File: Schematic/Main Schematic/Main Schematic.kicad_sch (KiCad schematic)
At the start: 5 parts, among them J1 Conn_01x10_Pin, J2 Conn_01x24_Socket, J3 Conn_01x24_Socket, SW2 SW_Push

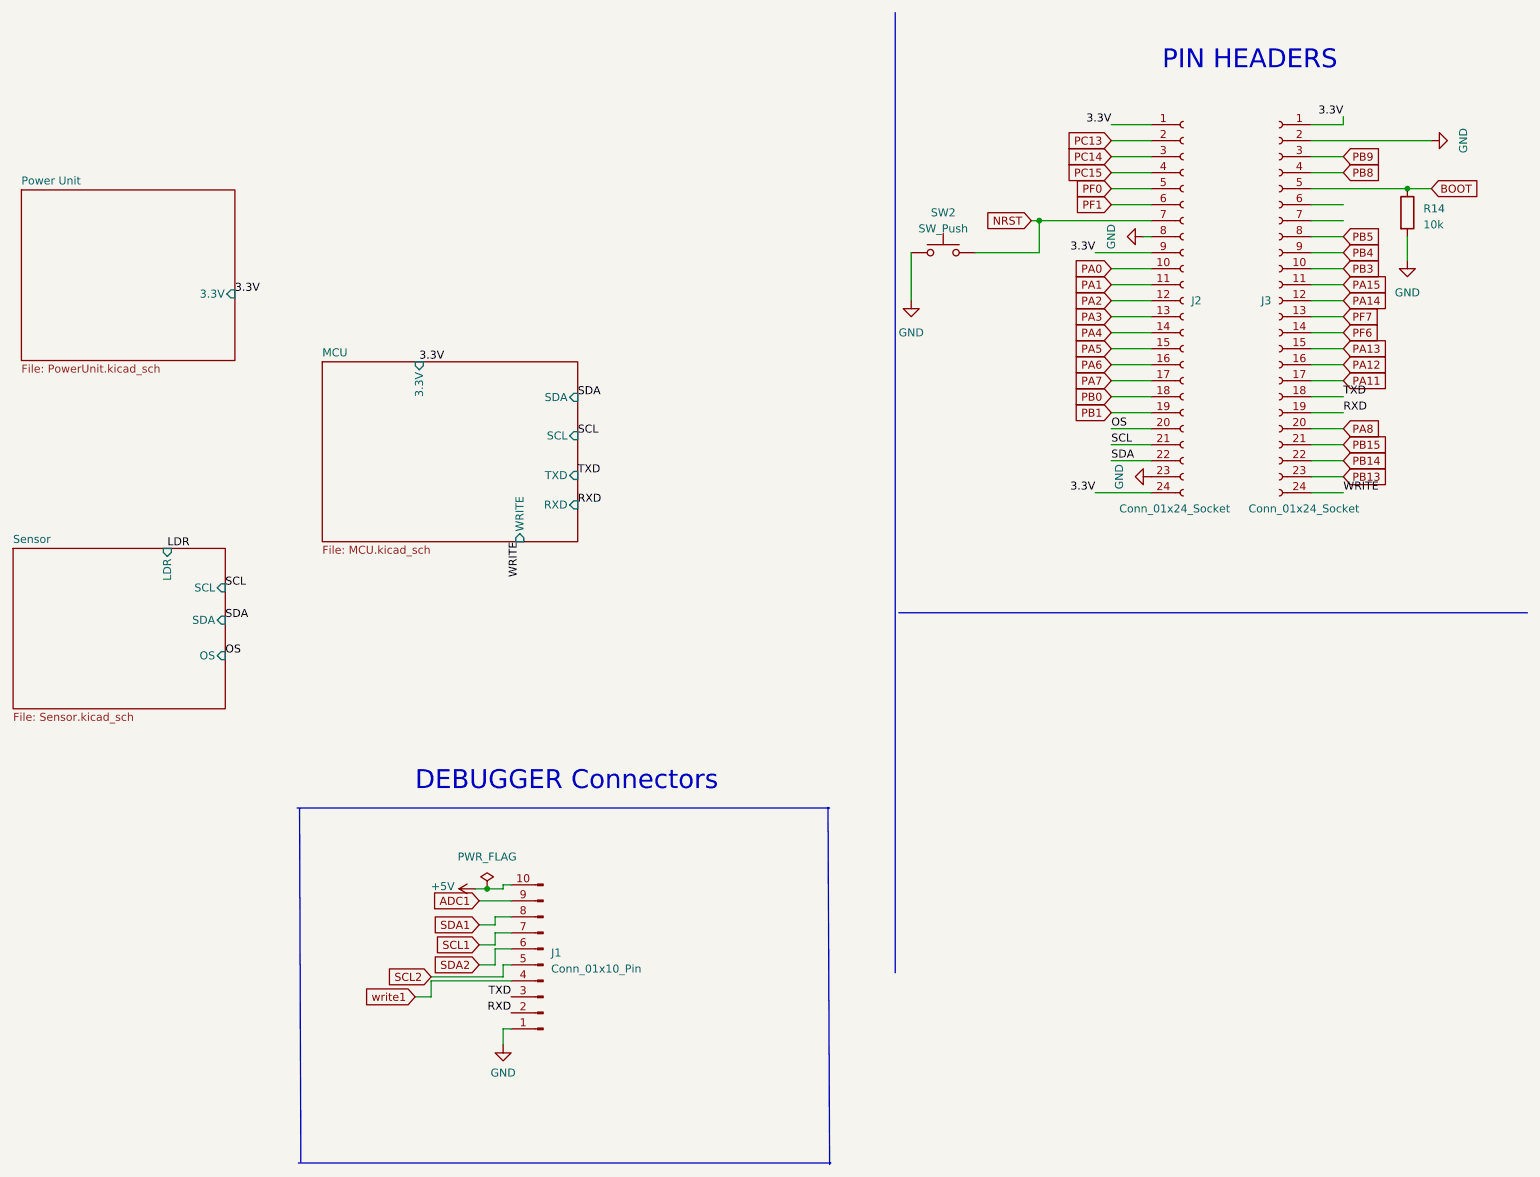
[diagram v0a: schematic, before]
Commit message: Update
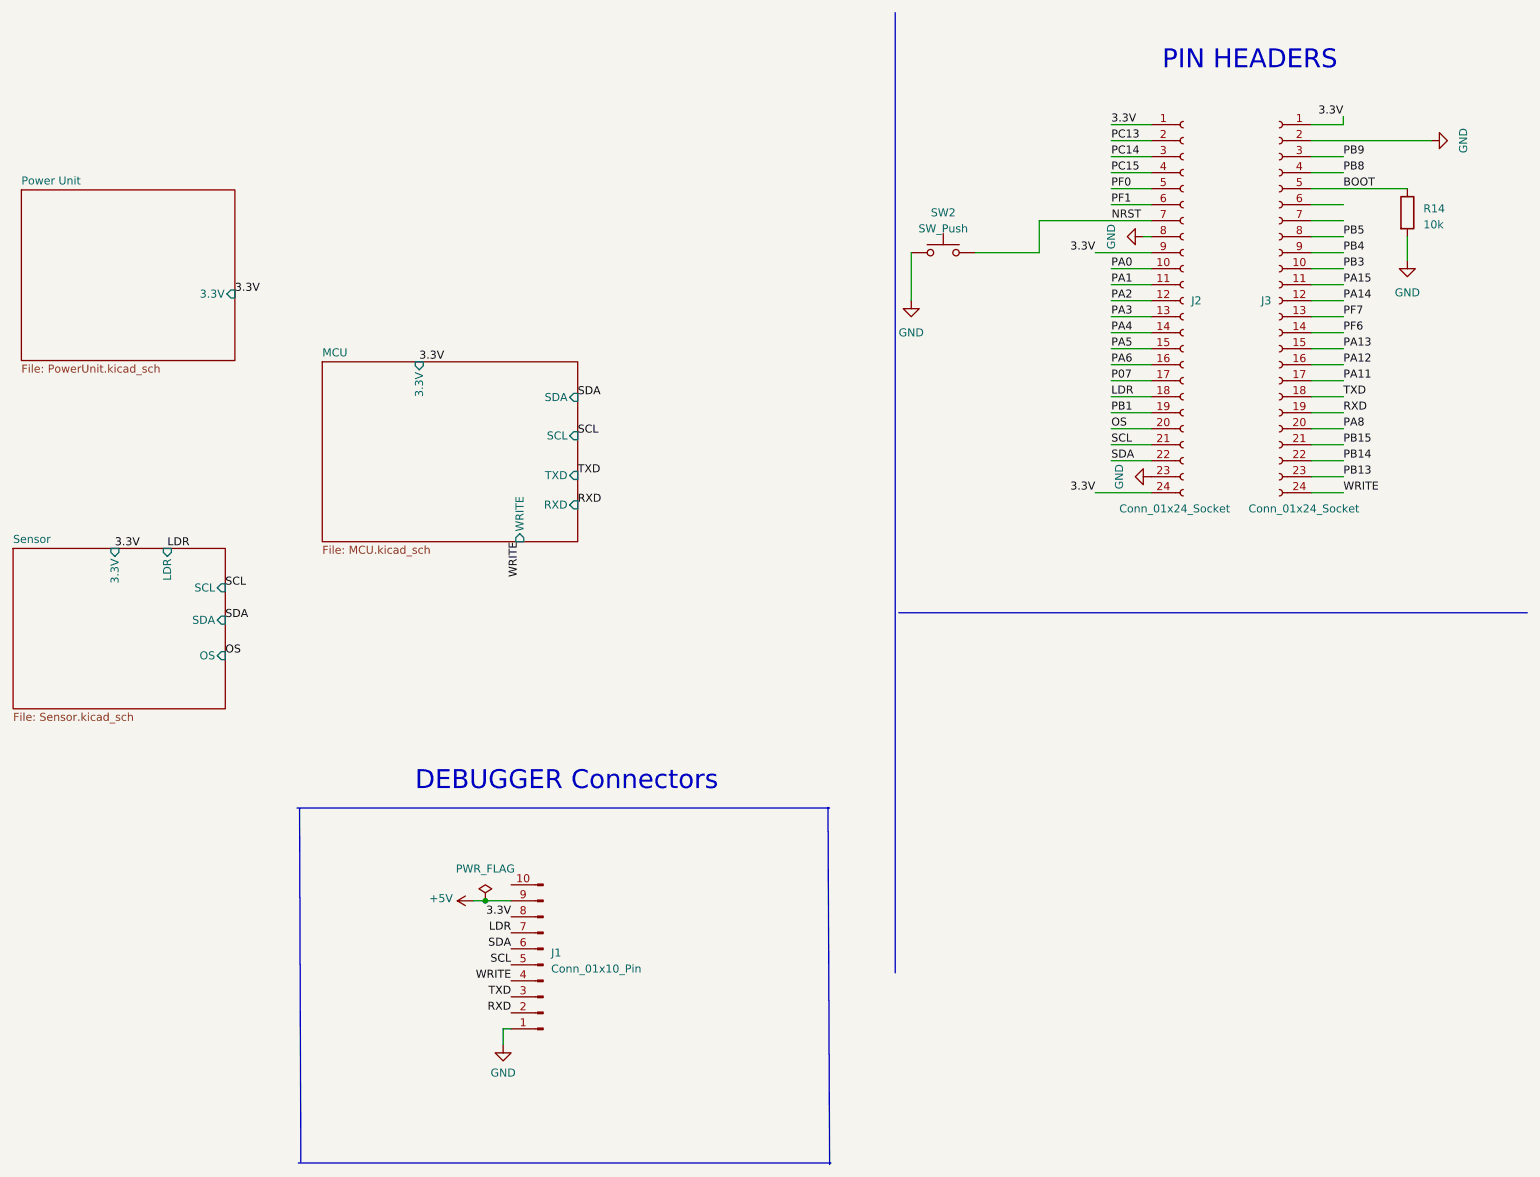
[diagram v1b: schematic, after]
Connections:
- net ADC1 is gone; now on net +5V: J1.9 (Pin_9)
- net PB0 is gone; now on net LDR: J2.18 (Pin_18)
- net SCL1 is gone; now on net LDR: J1.7 (Pin_7)
- net SCL2 is gone; now on net SCL: J1.5 (Pin_5)
- net SDA1 is gone; now on net 3.3V: J1.8 (Pin_8)
- net SDA2 is gone; now on net SDA: J1.6 (Pin_6)
- net write1 is gone; now on net WRITE: J1.4 (Pin_4)
- net +5V: no longer J1.10 (Pin_10)
- net PA7 renamed P07
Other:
- sheet Sensor ports: added 3.3V; removed none
